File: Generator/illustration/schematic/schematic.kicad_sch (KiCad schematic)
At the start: 9 parts, among them U1 ESP32 devkit v1, U2 LCD 16bit 2 lines 16pins, U3 6v-24v dc to 5v dc, U4 Hall effect sensor, U5 ESC 3 phase motor

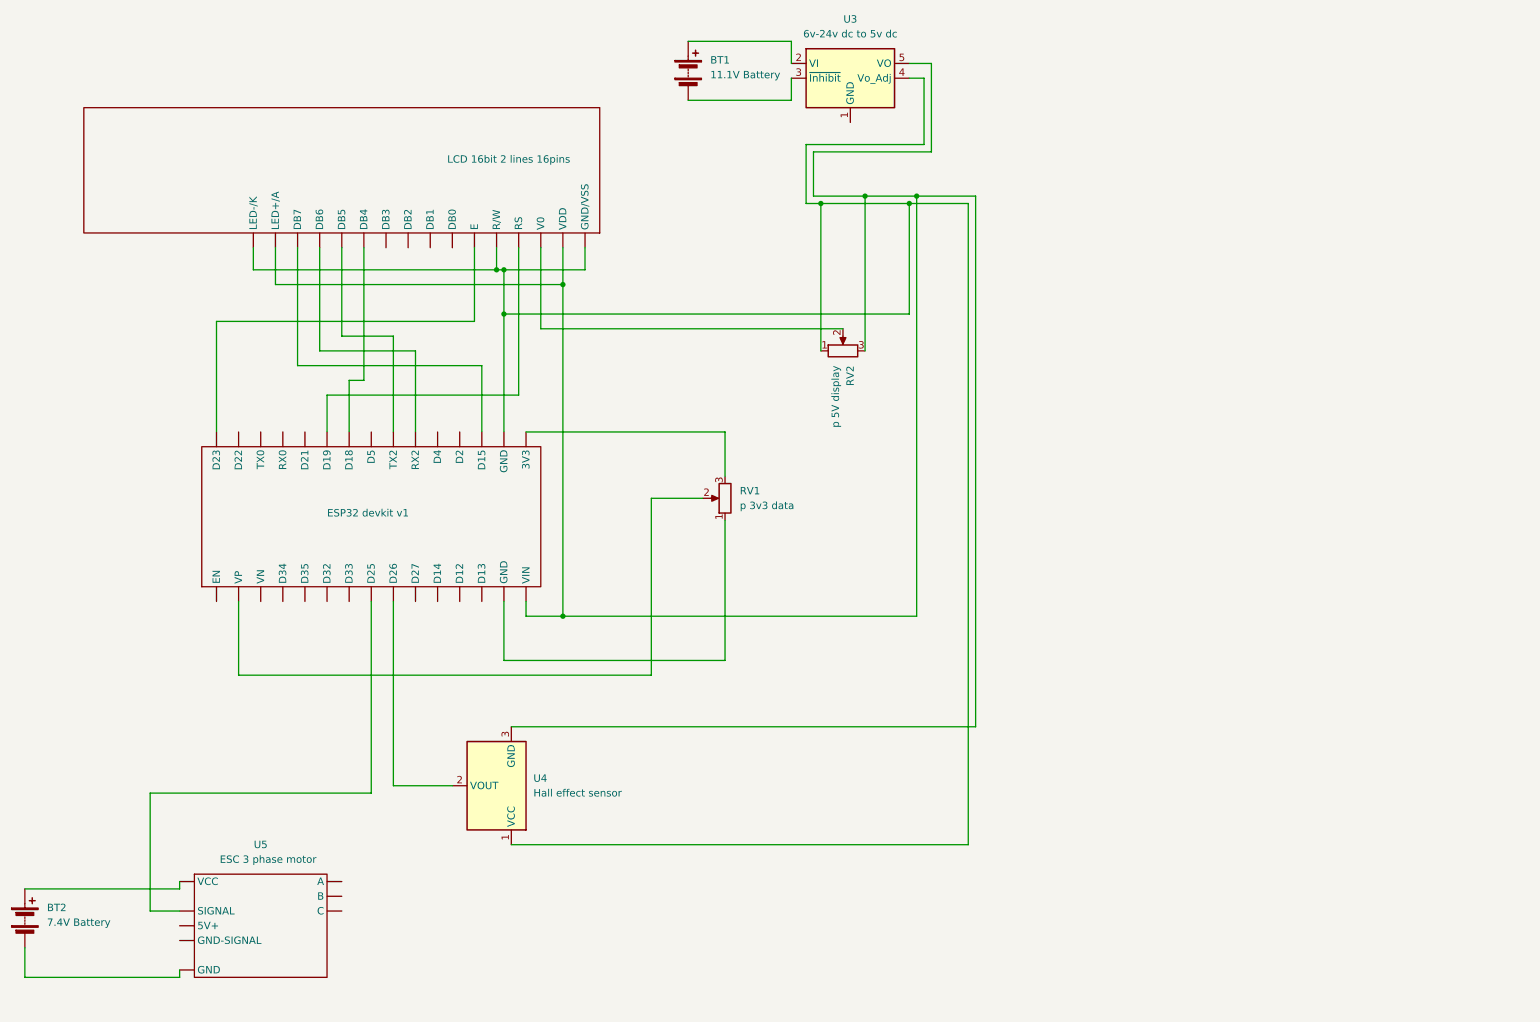
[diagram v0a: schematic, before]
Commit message: lezho
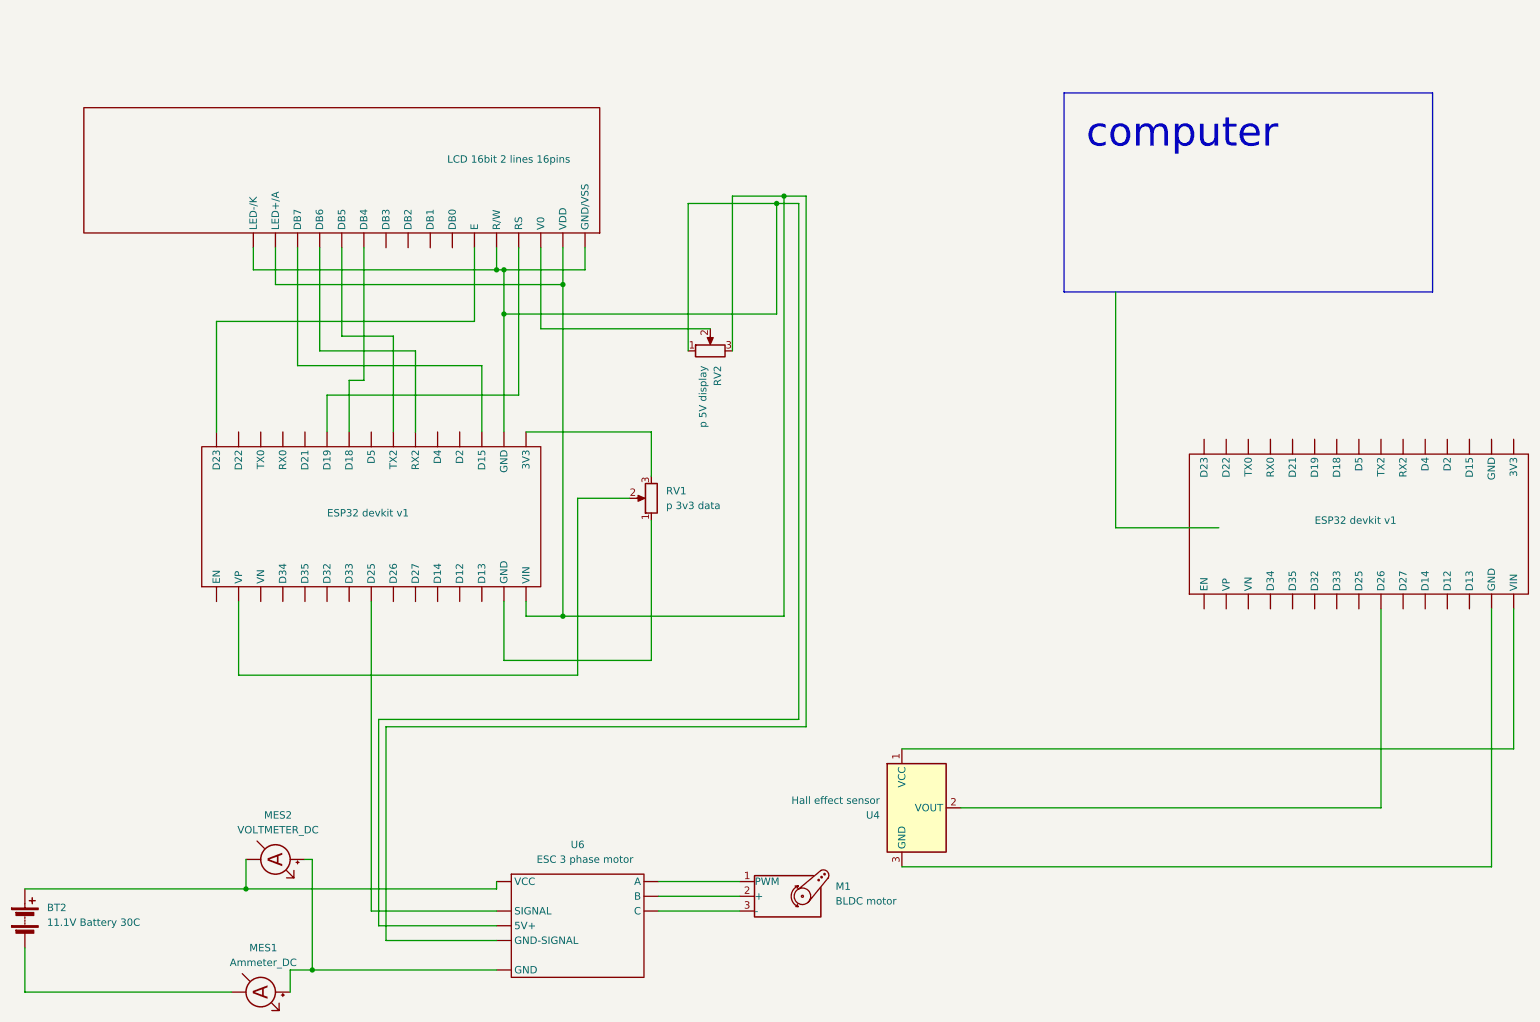
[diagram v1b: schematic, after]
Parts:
- removed BT1: 11.1V Battery, symbol Device:Battery
- removed U3: 6v-24v dc to 5v dc, Module:Texas_EUS_R-PDSS-T5_THT, symbol Converter_DCDC:PTN78000H_EUS-5
- removed U5: ESC 3 phase motor, Package_DIP:DIP-8_W10.16mm, symbol esc:esc
- added M1: BLDC motor, symbol Motor:Motor_Servo
- added MES1: Ammeter_DC, symbol Device:Ammeter_DC
- added MES2: VOLTMETER_DC, symbol Device:Ammeter_DC
- added U3: ESP32 devkit v1, Package_SO:TSSOP-30_6.1x9.7mm_P0.65mm, symbol esp32-30pins:ESP32
- added U6: ESC 3 phase motor, Package_DIP:DIP-8_W10.16mm, symbol esc:esc
- BT2: value 7.4V Battery -> 11.1V Battery 30C
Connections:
- net at U4.2 (VOUT): now also U3. (VP); no longer U1. (VP)
- net at U2. (VDD): now also RV2.2
- net at U1. (VP): now also RV1.3; no longer U2. (VDD)
- net at BT2.1 (+): now also MES2.1 (-), U6. (VCC)
- net at BT2.2 (-): now also MES1.1 (-)
- new net: M1.1 (PWM), U6. (VCC)
- new net: M1.2 (+), U6. (VCC)
- new net: M1.3 (-), U6. (VCC)
- new net: U3. (VP), U4.1 (VCC)
- new net: U3. (VP), U4.3 (GND)
- new net: MES1.2 (+), MES2.2 (+), U6. (VCC)
- new net: RV2.1, U1. (VP), U2. (VDD), U6. (VCC)
- new net: RV2.3, U1. (VP), U2. (VDD), U6. (VCC)
- new net: U1. (VP), U2. (VDD) (x6)
- new net: U1. (VP), U6. (VCC)
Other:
- moved on the sheet: RV1, RV2
